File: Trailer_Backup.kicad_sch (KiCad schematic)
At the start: 11 parts, among them Q36 IRLZ44N, SW6 SW_SPST, U10 LM339

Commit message: Add files via upload
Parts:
- R135: footprint Resistor_THT:R_Axial_DIN0207_L6.3mm_D2.5mm_P10.16mm_Horizontal -> PCM_SL_Devices:Resistor_5W
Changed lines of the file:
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@@
 			)
 		)
-		(property "Footprint" "Resistor_THT:R_Axial_DIN0207_L6.3mm_D2.5mm_P10.16mm_Horizontal"
+		(property "Footprint" "PCM_SL_Devices:Resistor_5W"
 			(at 94.869 65.278 0)
 			(hide yes)

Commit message: Add files via upload
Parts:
- R135: footprint PCM_SL_Devices:Resistor_5W -> Resistor_THT:R_Axial_Power_L25.0mm_W9.0mm_P27.94mm
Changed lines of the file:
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@@
 			)
 		)
-		(property "Footprint" "PCM_SL_Devices:Resistor_5W"
+		(property "Footprint" "Resistor_THT:R_Axial_Power_L25.0mm_W9.0mm_P27.94mm"
 			(at 94.869 65.278 0)
 			(hide yes)

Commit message: Add files via upload
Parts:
- R136, R137: footprint (none) -> TRIM_3296W1103LF:TRIM_3296W1103LF
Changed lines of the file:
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@@
 			)
 		)
-		(property "Footprint" ""
+		(property "Footprint" "TRIM_3296W1103LF:TRIM_3296W1103LF"
 			(at 100.33 50.8 0)
 			(hide yes)
@@
 			)
 		)
-		(property "Footprint" ""
+		(property "Footprint" "TRIM_3296W1103LF:TRIM_3296W1103LF"
 			(at 111.76 72.39 0)
 			(hide yes)

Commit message: Add files via upload
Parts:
- R135: footprint Resistor_THT:R_Axial_Power_L25.0mm_W9.0mm_P27.94mm -> Resistor_THT:R_Axial_DIN0207_L6.3mm_D2.5mm_P10.16mm_Horizontal
- R136, R137: footprint TRIM_3296W1103LF:TRIM_3296W1103LF -> (none)
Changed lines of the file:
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@@
 			)
 		)
-		(property "Footprint" "Resistor_THT:R_Axial_Power_L25.0mm_W9.0mm_P27.94mm"
+		(property "Footprint" "Resistor_THT:R_Axial_DIN0207_L6.3mm_D2.5mm_P10.16mm_Horizontal"
 			(at 94.869 65.278 0)
 			(hide yes)
@@
 			)
 		)
-		(property "Footprint" "TRIM_3296W1103LF:TRIM_3296W1103LF"
+		(property "Footprint" ""
 			(at 100.33 50.8 0)
 			(hide yes)
@@
 			)
 		)
-		(property "Footprint" "TRIM_3296W1103LF:TRIM_3296W1103LF"
+		(property "Footprint" ""
 			(at 111.76 72.39 0)
 			(hide yes)

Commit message: Add files via upload
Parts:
- R135: footprint Resistor_THT:R_Axial_DIN0207_L6.3mm_D2.5mm_P10.16mm_Horizontal -> Resistor_THT:R_Axial_Power_L25.0mm_W9.0mm_P27.94mm
- R136, R137: footprint (none) -> TRIM_3296W1103LF:TRIM_3296W1103LF
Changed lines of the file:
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@@
 			)
 		)
-		(property "Footprint" "Resistor_THT:R_Axial_DIN0207_L6.3mm_D2.5mm_P10.16mm_Horizontal"
+		(property "Footprint" "Resistor_THT:R_Axial_Power_L25.0mm_W9.0mm_P27.94mm"
 			(at 94.869 65.278 0)
 			(hide yes)
@@
 			)
 		)
-		(property "Footprint" ""
+		(property "Footprint" "TRIM_3296W1103LF:TRIM_3296W1103LF"
 			(at 100.33 50.8 0)
 			(hide yes)
@@
 			)
 		)
-		(property "Footprint" ""
+		(property "Footprint" "TRIM_3296W1103LF:TRIM_3296W1103LF"
 			(at 111.76 72.39 0)
 			(hide yes)

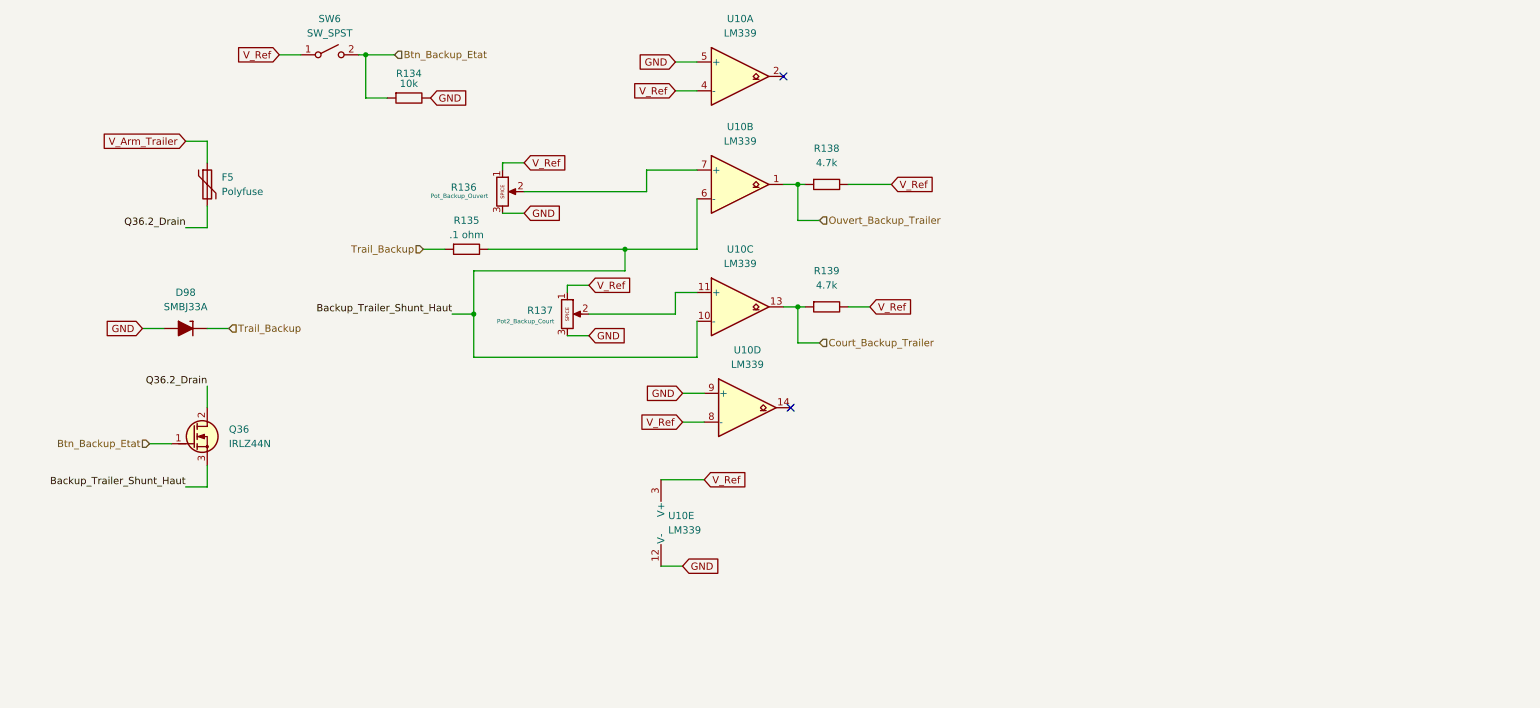
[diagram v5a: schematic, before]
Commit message: Add files via upload
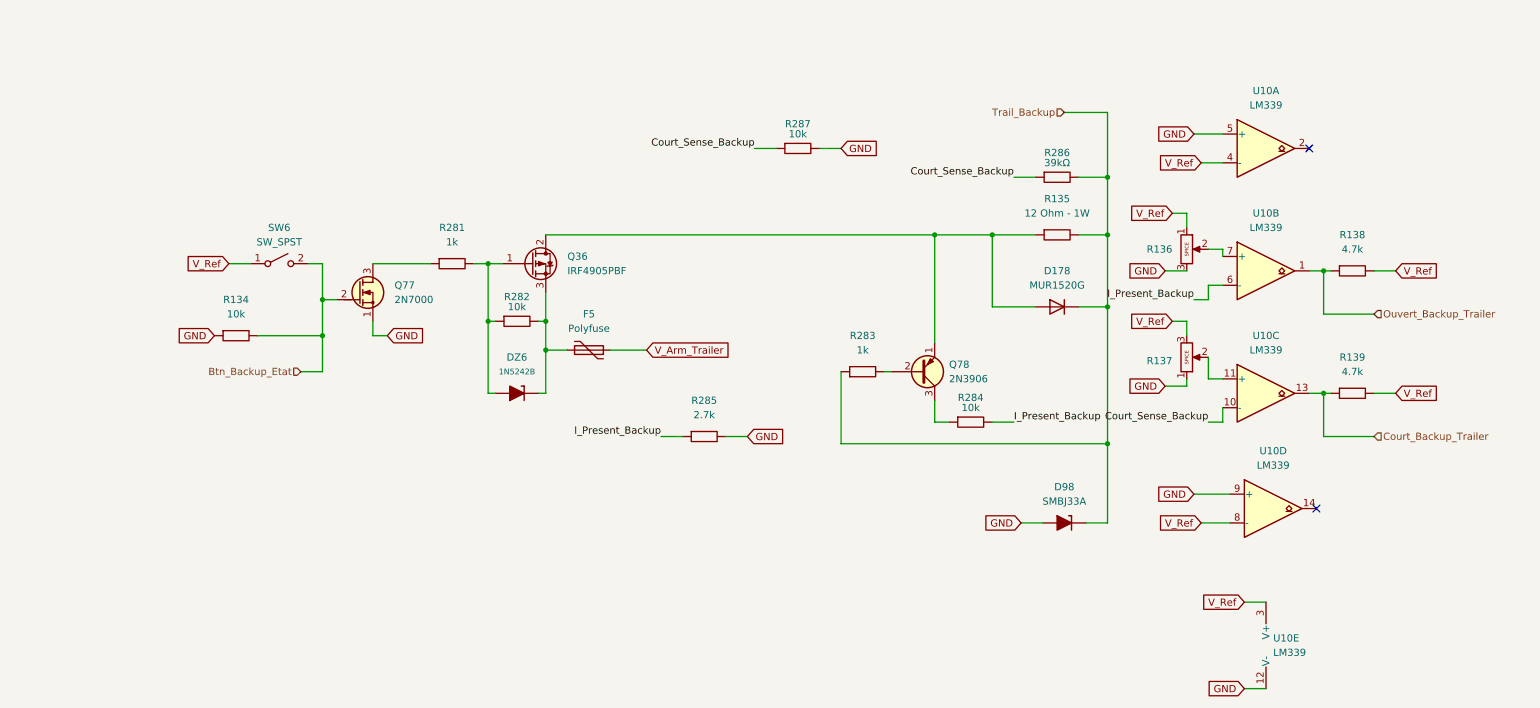
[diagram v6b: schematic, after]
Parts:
- removed Q36: IRLZ44N, PCM_Package_TO_SOT_THT_AKL:TO-220-3_Vertical_GDS, symbol PCM_Transistor_MOSFET_AKL:IRLZ44N
- removed R134: 10k, Resistor_THT:R_Axial_DIN0207_L6.3mm_D2.5mm_P10.16mm_Horizontal, symbol PCM_SL_Resistors:10k
- removed R135: .1 ohm, Resistor_THT:R_Axial_Power_L25.0mm_W9.0mm_P27.94mm, symbol PCM_SL_Resistors:4.7k
- added D178: MUR1520G, Package_TO_SOT_THT:TO-220-2_Vertical, symbol Device:D
- added DZ6: 1N5242B, PCM_Diode_THT_AKL:D_DO-35_SOD27_P7.62mm_Horizontal_Zener, symbol PCM_Diode_Zener_AKL:1N5242B
- added Q36: IRF4905PBF, Package_TO_SOT_THT:TO-220-3_Vertical, symbol Transistor_FET:IRF4905
- added Q77: 2N7000, PCM_Package_TO_SOT_THT_AKL:TO-92_Inline_Wide_SGD, symbol PCM_Transistor_MOSFET_AKL:2N7000
- added Q78: 2N3906, PCM_Package_TO_SOT_THT_AKL:TO-92_Inline_Wide_EBC, symbol PCM_Transistor_BJT_AKL:2N3906
- added R134: 10k, Resistor_THT:R_Axial_DIN0207_L6.3mm_D2.5mm_P10.16mm_Horizontal, symbol PCM_SL_Resistors:4.7k
- added R135: 12 Ohm - 1W, Resistor_THT:R_Axial_DIN0414_L11.9mm_D4.5mm_P15.24mm_Horizontal, symbol PCM_SL_Devices:Resistor_5W
- added R281, R283: 1k, Resistor_THT:R_Axial_DIN0207_L6.3mm_D2.5mm_P10.16mm_Horizontal, symbol PCM_SL_Resistors:1k
- added R282, R284, R287: 10k, Resistor_THT:R_Axial_DIN0207_L6.3mm_D2.5mm_P10.16mm_Horizontal, symbol PCM_SL_Resistors:10k
- added R285: 2.7k, Resistor_THT:R_Axial_DIN0207_L6.3mm_D2.5mm_P10.16mm_Horizontal, symbol PCM_SL_Resistors:2.7k
- added R286: 39kΩ, Resistor_THT:R_Axial_DIN0207_L6.3mm_D2.5mm_P10.16mm_Horizontal, symbol PCM_SL_Resistors:10k
- R136: Etiquette Pot_Backup_Ouvert -> (none)
- R137: Etiquette Pot2_Backup_Court -> (none)
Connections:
- net Btn_Backup_Etat: now also Q77.2 (G), R134.2
- net GND: now also R137.1, Q77.1 (S), R134.1, R285.2, R287.2; no longer R137.3
- net Trail_Backup: now also D178.1 (K), R135.2, R283.1, R286.2
- net V_Ref: now also R137.3; no longer R137.1
- net Backup_Trailer_Shunt_Haut renamed Court_Sense_Backup
- net Court_Sense_Backup: now also R286.1, R287.1; no longer U10.6 (-)
- net Q36.2_Drain: no longer names the net of F5.2
- net Q36.2_Drain: now also DZ6.1 (K), Q36.3 (S), R282.2
- new net: DZ6.2 (A), Q36.1 (G), R281.2, R282.1
- new net: D178.2 (A), Q36.2 (D), Q78.1 (E), R135.1
- new net: Q77.3 (D), R281.1
- new net: Q78.2 (B), R283.2
- new net: Q78.3 (C), R284.1
- new net I_Present_Backup: R284.2, R285.1, U10.6 (-)
